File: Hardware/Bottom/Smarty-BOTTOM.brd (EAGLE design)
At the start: 33 x 33 mm, 36 parts, among them U4 PCF8523

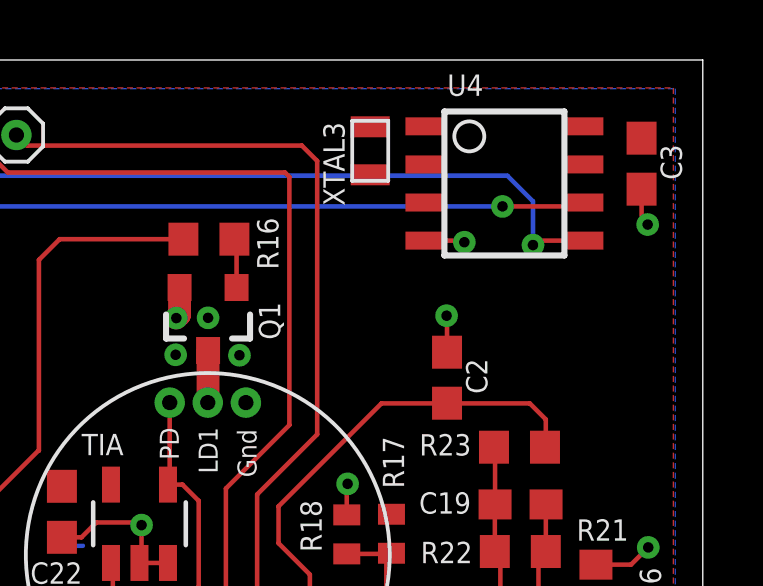
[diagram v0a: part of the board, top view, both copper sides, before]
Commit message: Finished Take 008
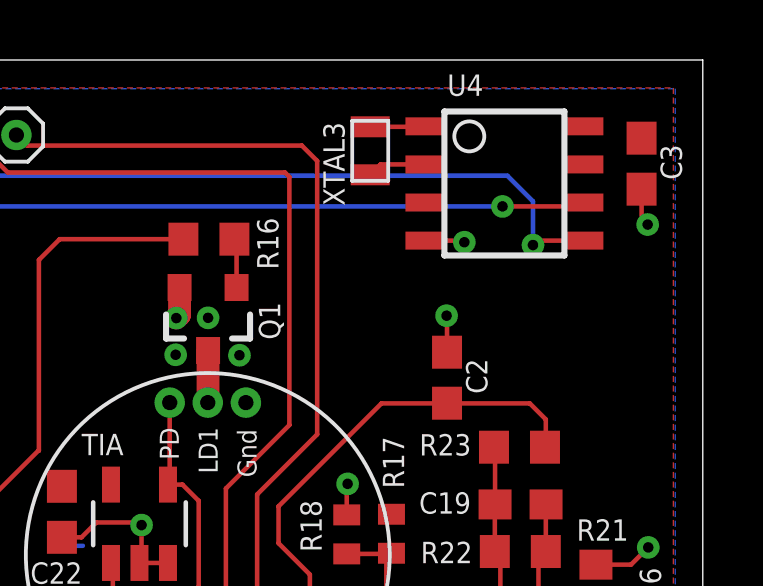
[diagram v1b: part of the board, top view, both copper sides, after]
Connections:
- net N$1: now also XTAL3.P$1
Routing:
- net N$1: track 0.00 -> 1.97 mm
- net N$2: track 0.00 -> 1.83 mm
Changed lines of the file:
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@@
 <wire x1="22.402803125" y1="18.34895625" x2="21.358859375" y2="19.3929" width="0.1524" layer="1"/>
 <wire x1="21.358859375" y1="19.3929" x2="21.358859375" y2="20.6222625" width="0.1524" layer="1"/>
-<wire x1="24.790396875" y1="24.0538" x2="29.733240625" y2="24.0538" width="0.1524" layer="1"/>
+<wire x1="24.790396875" y1="24.0538" x2="26.990040625" y2="24.0538" width="0.1524" layer="1"/>
+<wire x1="26.990040625" y1="24.0538" x2="29.733240625" y2="24.0538" width="0.1524" layer="1"/>
 <wire x1="29.733240625" y1="24.0538" x2="30.266640625" y2="23.5204" width="0.1524" layer="1"/>
 <wire x1="30.266640625" y1="22.619596875" x2="30.240340625" y2="22.593296875" width="0.1524" layer="1"/>
@@
 <wire x1="24.942803125" y1="13.334996875" x2="24.942803125" y2="11.634159375" width="0.1524" layer="1"/>
 <contactref element="C2" pad="2"/>
-<wire x1="30.240340625" y1="22.593296875" x2="26.9748" y2="24.059778125" width="0" layer="19" extent="1-1"/>
+<wire x1="26.9748" y1="24.059778125" x2="26.9840625" y2="24.059778125" width="0.1524" layer="1"/>
+<wire x1="26.9840625" y1="24.059778125" x2="26.990040625" y2="24.0538" width="0.1524" layer="1"/>
 </signal>
 <signal name="N$9">
@@
 <signal name="N$1">
 <contactref element="U4" pad="2"/>
+<contactref element="XTAL3" pad="P$1"/>
+<wire x1="24.414475" y1="31.673896875" x2="24.75981875" y2="32.019240625" width="0.1524" layer="1"/>
+<wire x1="24.75981875" y1="32.019240625" x2="26.23741875" y2="32.019240625" width="0.1524" layer="1"/>
 </signal>
 <signal name="N$2">
 <contactref element="XTAL3" pad="P$2"/>
 <contactref element="U4" pad="1"/>
-<wire x1="24.414475" y1="33.273896875" x2="26.23741875" y2="33.289240625" width="0" layer="19" extent="1-1"/>
+<wire x1="26.23741875" y1="33.289240625" x2="26.222075" y2="33.273896875" width="0.1524" layer="1"/>
+<wire x1="26.222075" y1="33.273896875" x2="24.414475" y2="33.273896875" width="0.1524" layer="1"/>
 </signal>
 </signals>
